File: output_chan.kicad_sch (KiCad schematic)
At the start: 11 parts, among them U4 MAX14917AFM+

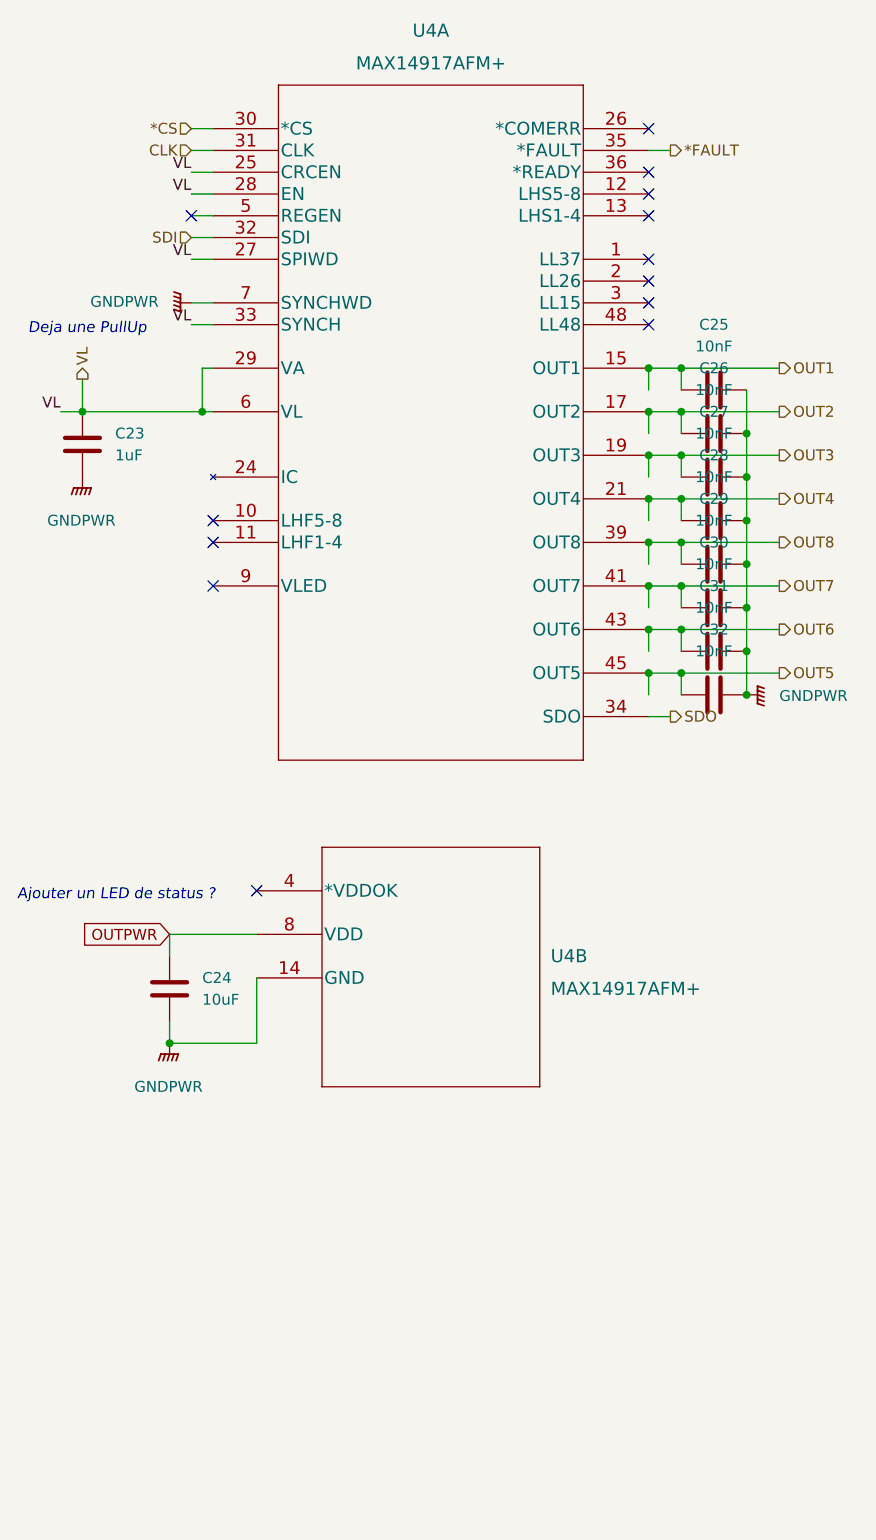
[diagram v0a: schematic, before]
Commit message: fix warnings
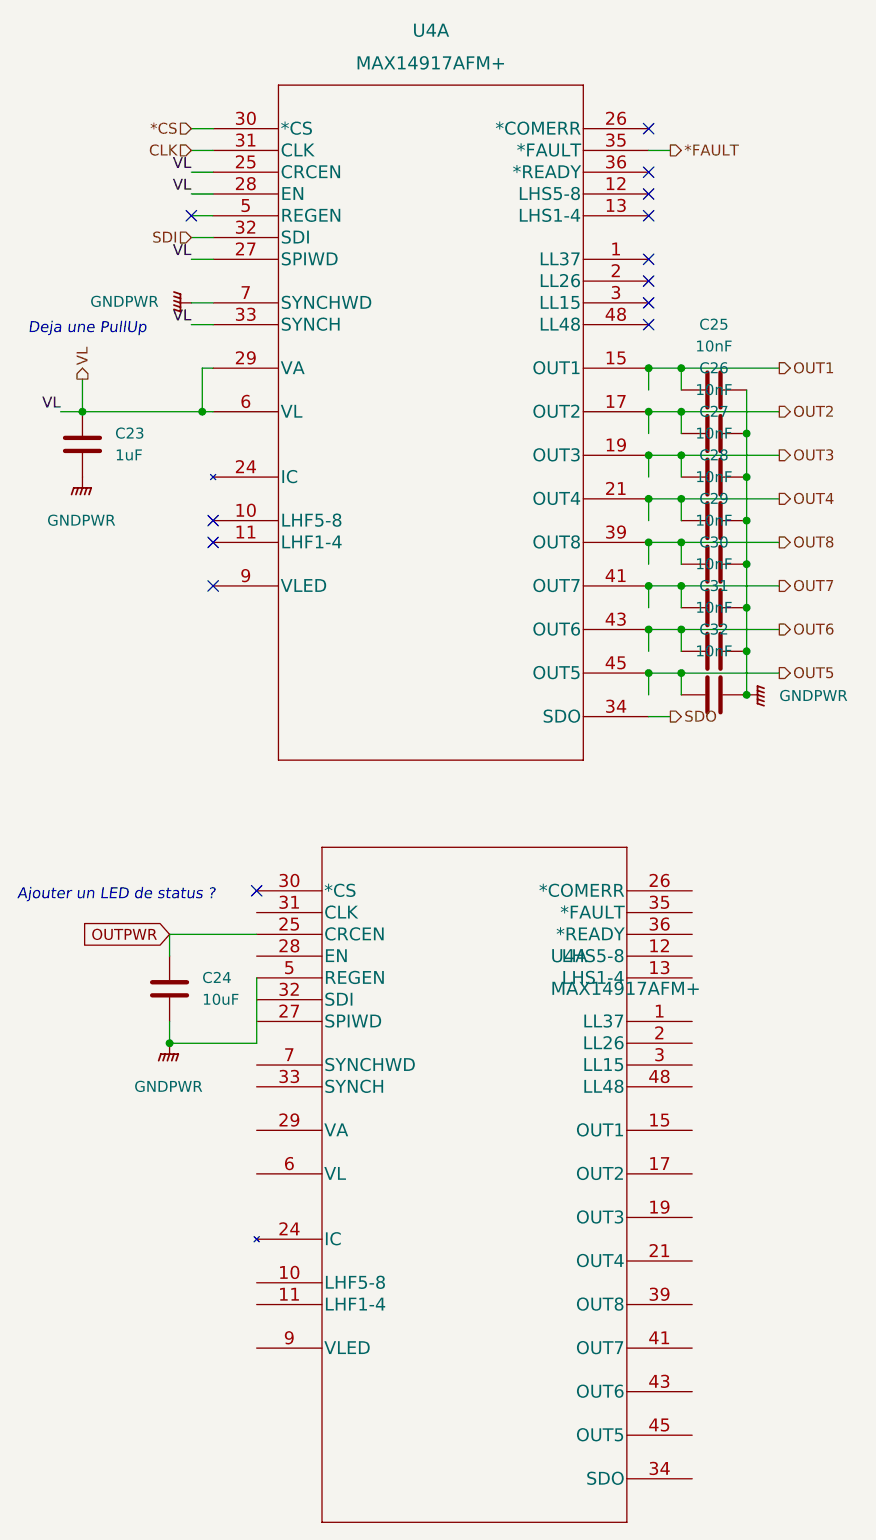
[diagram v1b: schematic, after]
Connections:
- net GNDPWR: now also U4.5 (REGEN); no longer U4.14 (GND), U4.23 (GND), U4.38 (GND), U4.47 (GND)
- net OUTPWR: now also U4.25 (CRCEN); no longer U4.49 (EPAD), U4.8 (VDD)
- new net: U4.15 (OUT1), U4.16 (OUT1)
- new net: U4.17 (OUT2), U4.18 (OUT2)
- new net: U4.19 (OUT3), U4.20 (OUT3)
- new net: U4.21 (OUT4), U4.22 (OUT4)
- new net: U4.37 (VL), U4.6 (VL)
- new net: U4.39 (OUT8), U4.40 (OUT8)
- new net: U4.41 (OUT7), U4.42 (OUT7)
- new net: U4.43 (OUT6), U4.44 (OUT6)
- new net: U4.45 (OUT5), U4.46 (OUT5)
